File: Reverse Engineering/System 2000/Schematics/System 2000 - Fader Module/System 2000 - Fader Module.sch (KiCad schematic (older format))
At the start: 29 parts, among them J10 CONN 1X2, J12 CONN 1X2, J3 802, J4 556 ?, J6 501, M2.1 OO PAD, U4 LM78L05ACZ/NOPB, U5 TLC27L4AIN, U7 LM78L05ACZ/NOPB

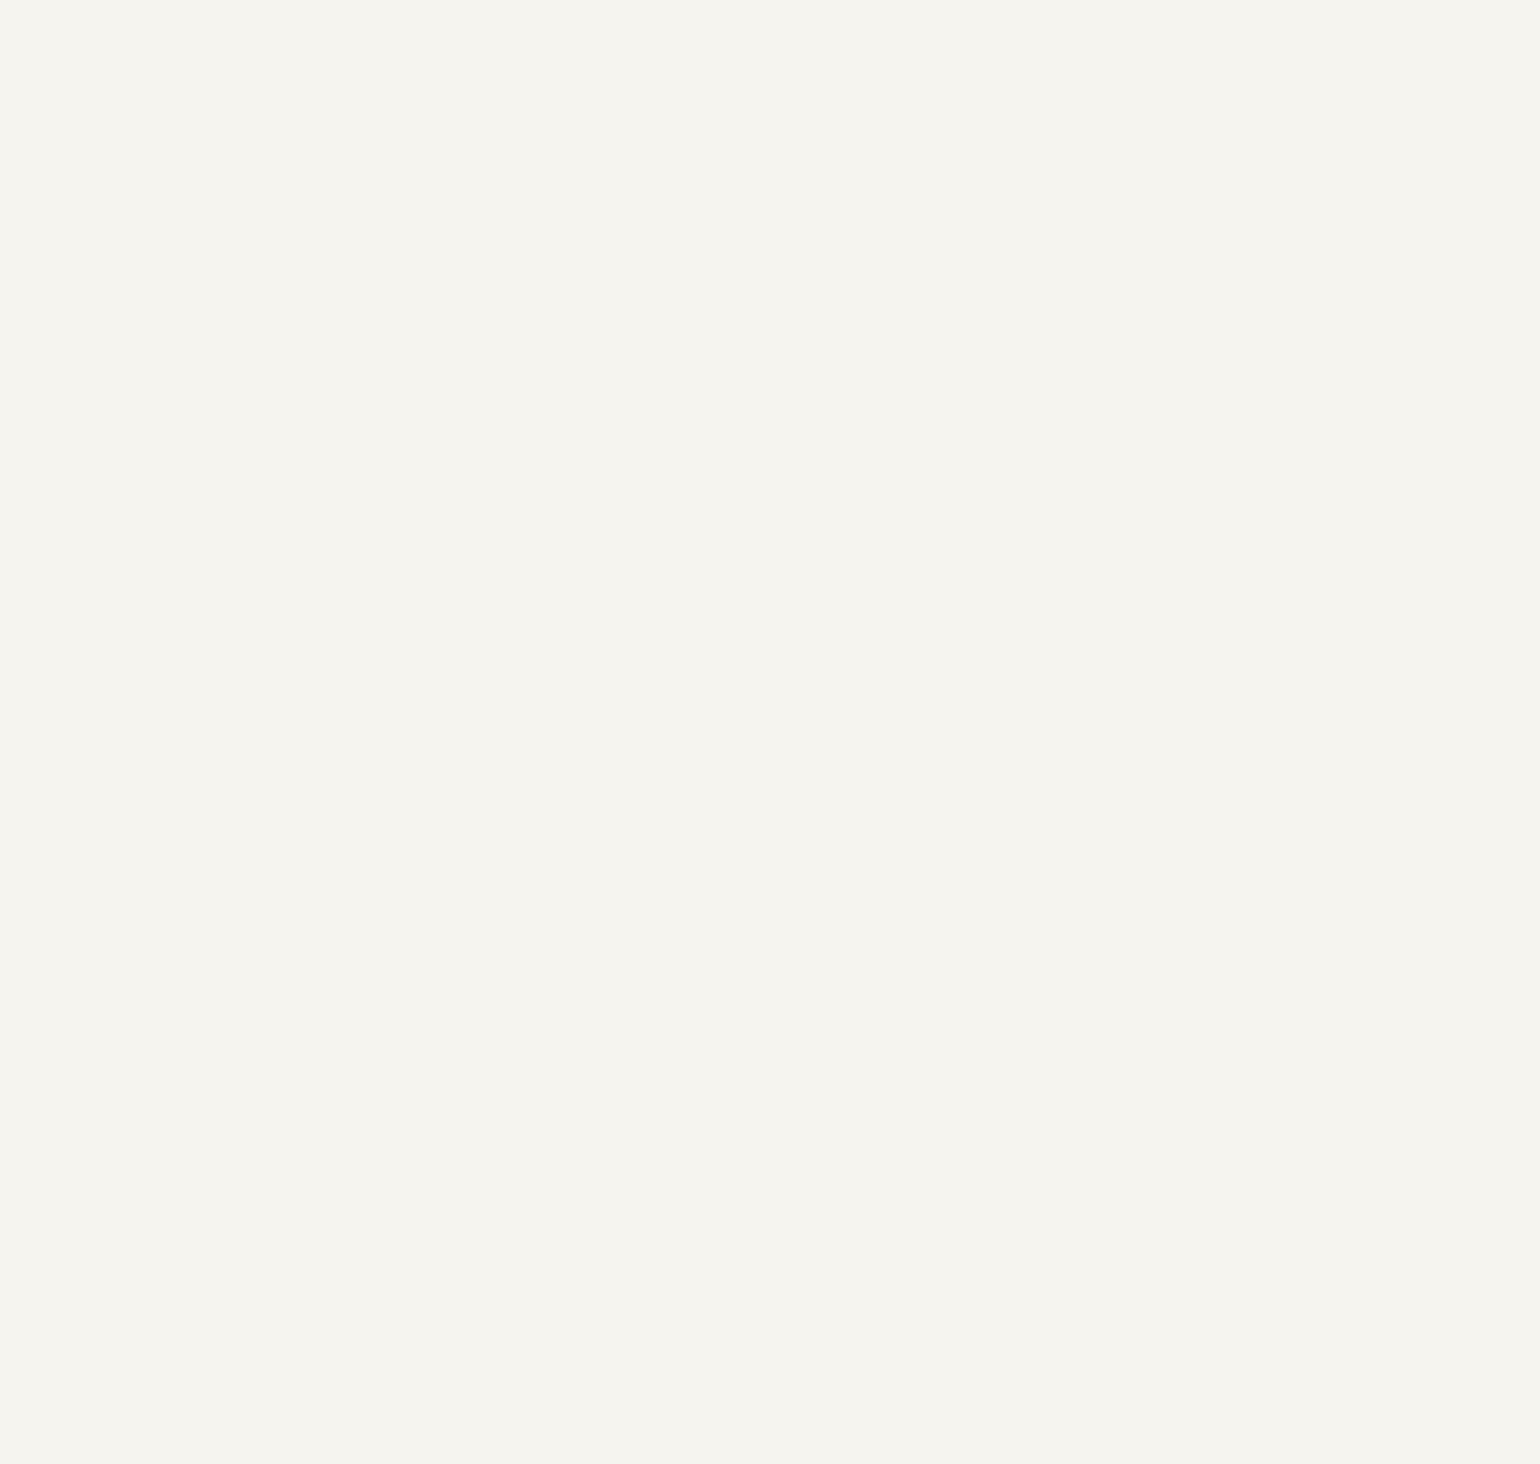
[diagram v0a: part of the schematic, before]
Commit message: 0.1.1
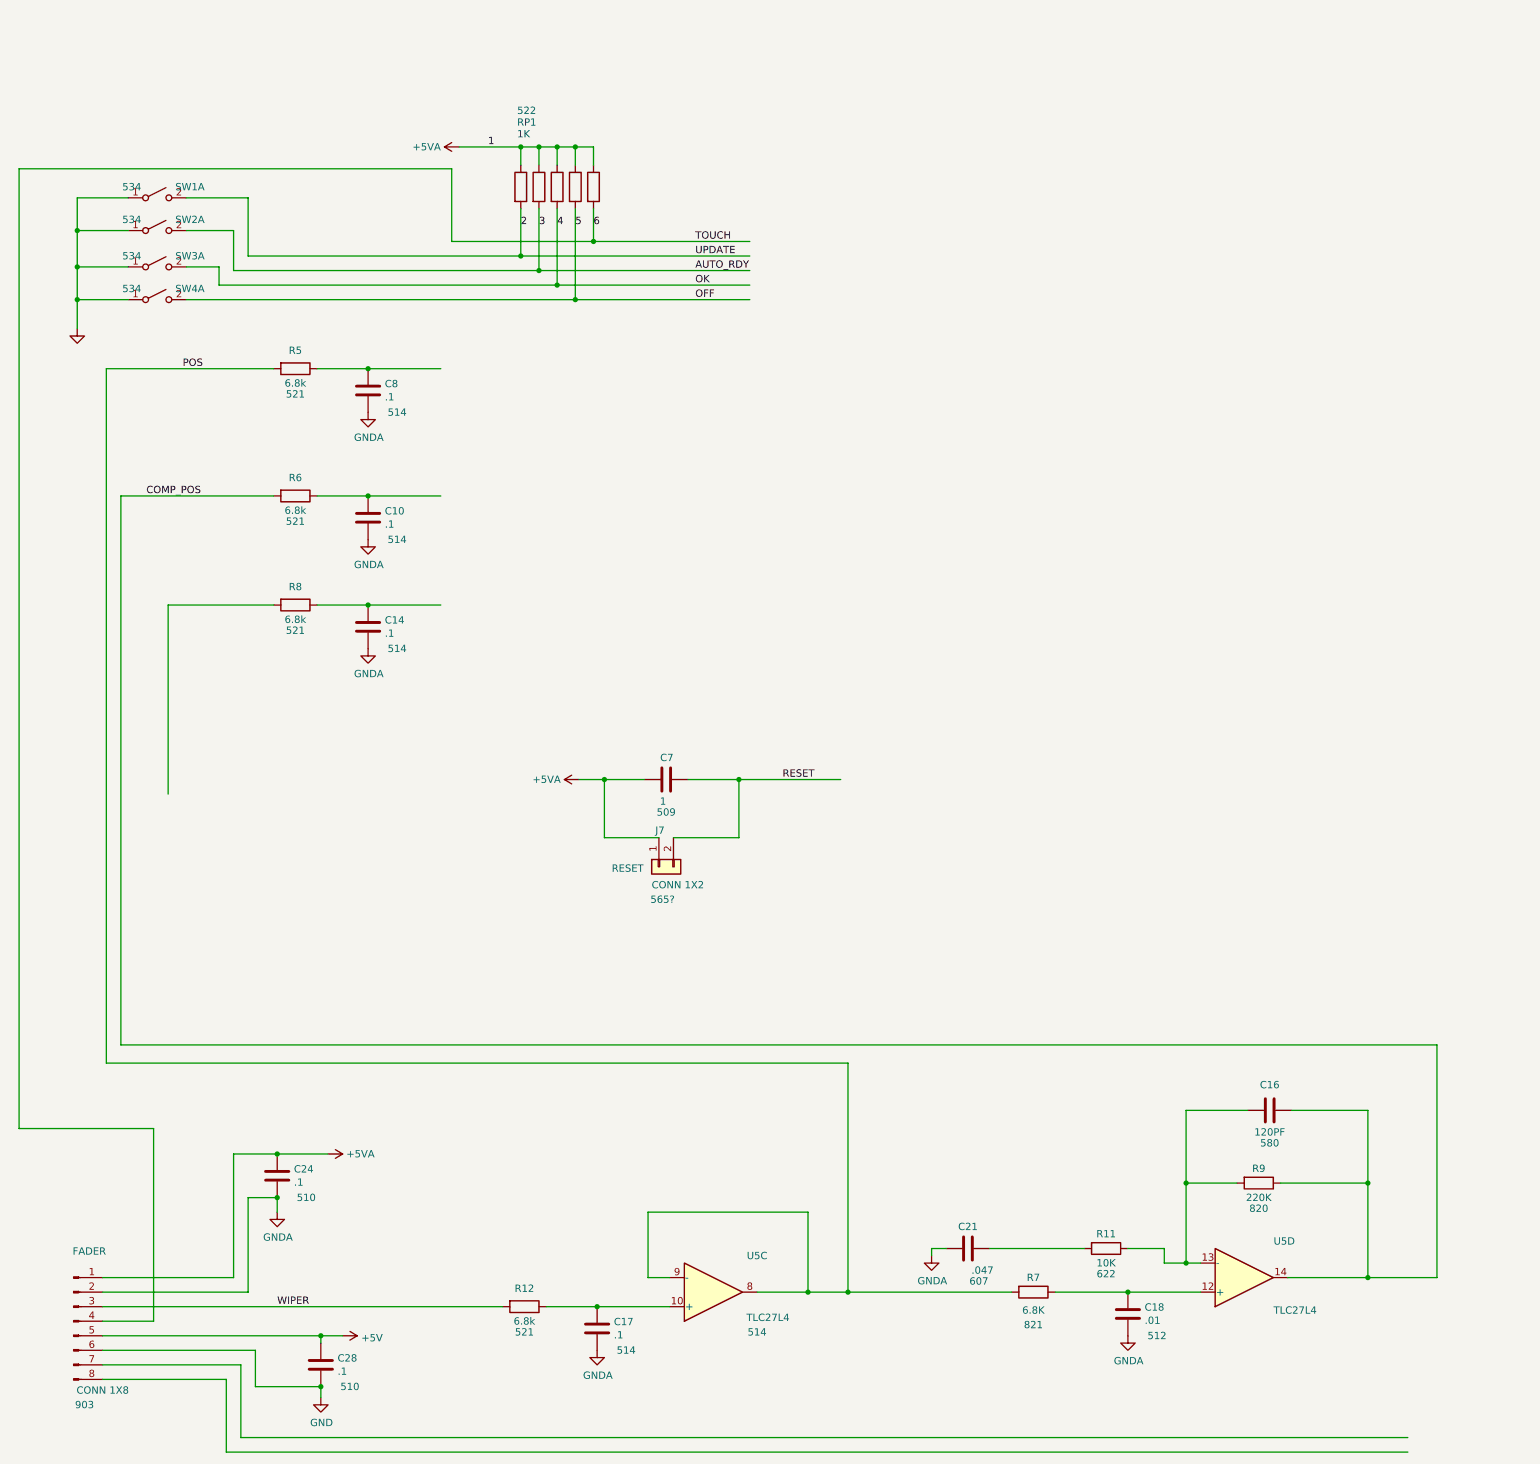
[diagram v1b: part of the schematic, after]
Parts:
- added C10, C14, C17, C24, C28, C8: .1, symbol Device:C
- added C16: 120PF, symbol Device:C
- added C18: .01, symbol Device:C
- added C21: .047, symbol Device:C
- added C7: 1, symbol Device:C
- added FADER: CONN 1X8, symbol Connector:Conn_01x08_Male
- added J7: CONN 1X2, symbol Connector_Generic:Conn_01x02
- added R11: 10K, symbol Device:R
- added R12, R5, R6, R8: 6.8k, symbol Device:R
- added R7: 6.8K, symbol Device:R
- added R9: 220K, symbol Device:R
- added R? (x5): 1K, symbol Device:R
- added SW1, SW2, SW3, SW4: SW_DPST_x2, symbol Switch:SW_DPST_x2
- added unit 3 of U5
- added unit 4 of U5
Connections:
- net labels added: +5VA, 1, 2, 3, 4, 5, 6, AUTO_RDY, COMP_POS, GNDA, OFF, OK, POS, RESET, TOUCH, UPDATE, WIPER
- wire segments 131 -> 250
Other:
- note added: "522\nRP1\n1K"
- note added: "RESET"

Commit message: 0.1.1.1
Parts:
- added C3, C5: 27PF, symbol Device:C
- added D1, D? (x4): LED, symbol Device:LED
- added ISO1, ISO2, ISO3, ISO4, U?: CNY17-3, symbol Isolator:CNY17-3
- added J1: CONN 1X10, symbol Connector_Generic:Conn_01x10
- added J11: CONN 4, symbol Connector:Conn_01x04_Male
- added J8: CONN 2X4, symbol Connector_Generic:Conn_02x04_Odd_Even
- added R1: 2K, symbol Device:R
- added R2, R? (x10): 1K, symbol Device:R
- added R3, R4: 100, symbol Device:R
- added X1: 12.000MHZ, symbol Device:Crystal
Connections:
- net labels added: +(RED), -(RED), AUTO(GRN), ON_OFF(RED), READY(YEL), RX, TX
- wire segments 250 -> 417
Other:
- note added: "OPTO I/O"
- note added: "RP1\n1K\n522"
- note added: "SWITCH BANK 1"
- note added: "SWITCH BANK 2"
- note added: "SWITCH BANK 3"
- note added: "SWITCH BANK 4"
- note added: "TEST OPTION"
- moved on the sheet: C10, C14, C16, C17, C18, C21, C24, C28, C7, C8, FADER, J6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
